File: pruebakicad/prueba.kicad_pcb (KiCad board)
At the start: 2 copper layers, 37 parts, among them J1 Conn_01x08_RC522, J2 Conn_01x04_MountingPin, J3 Conn_01x03, J4 Conn_2Rows-15Pins, J5 Conn_01x04, J6 Conn_01x02, Q1 BSS138, Q2 BSS138, U1 TLV1117-33, U2 TLV1117-50, U3 ESP32-WROOM-32

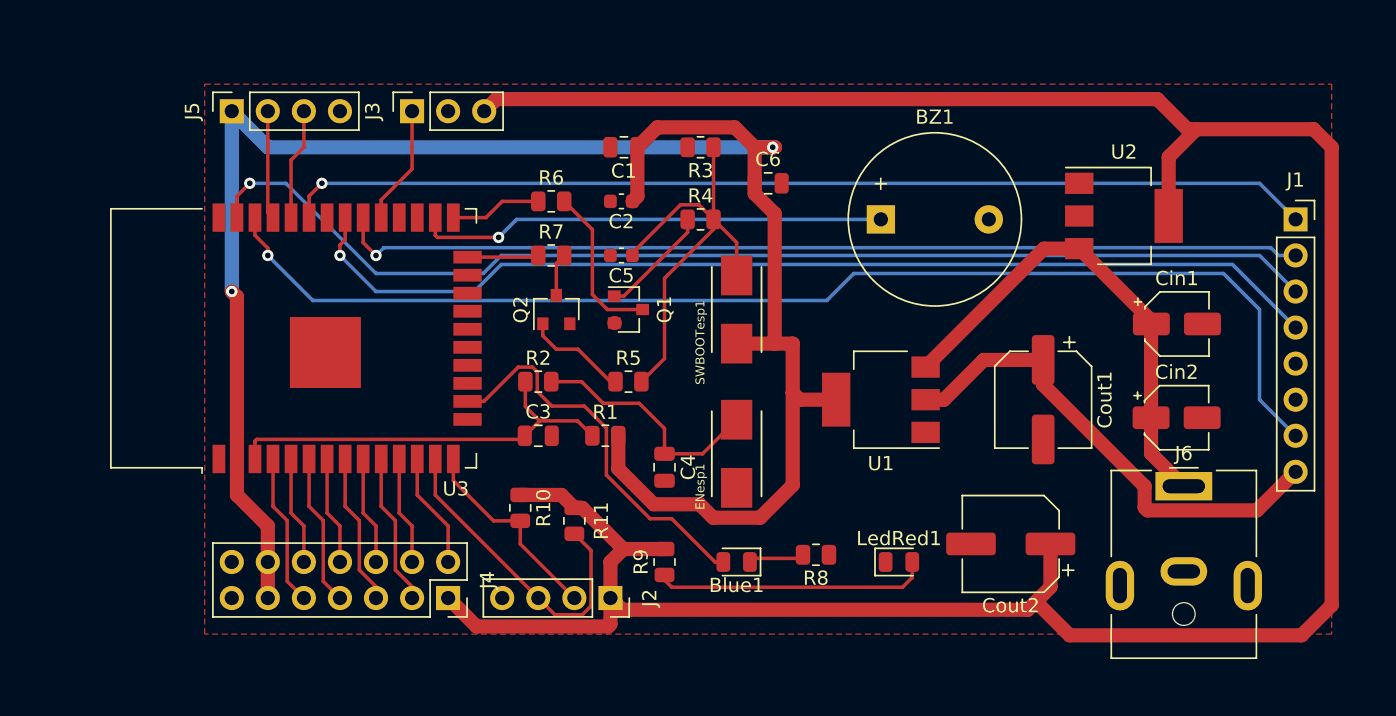
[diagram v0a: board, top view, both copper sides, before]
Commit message: tierras
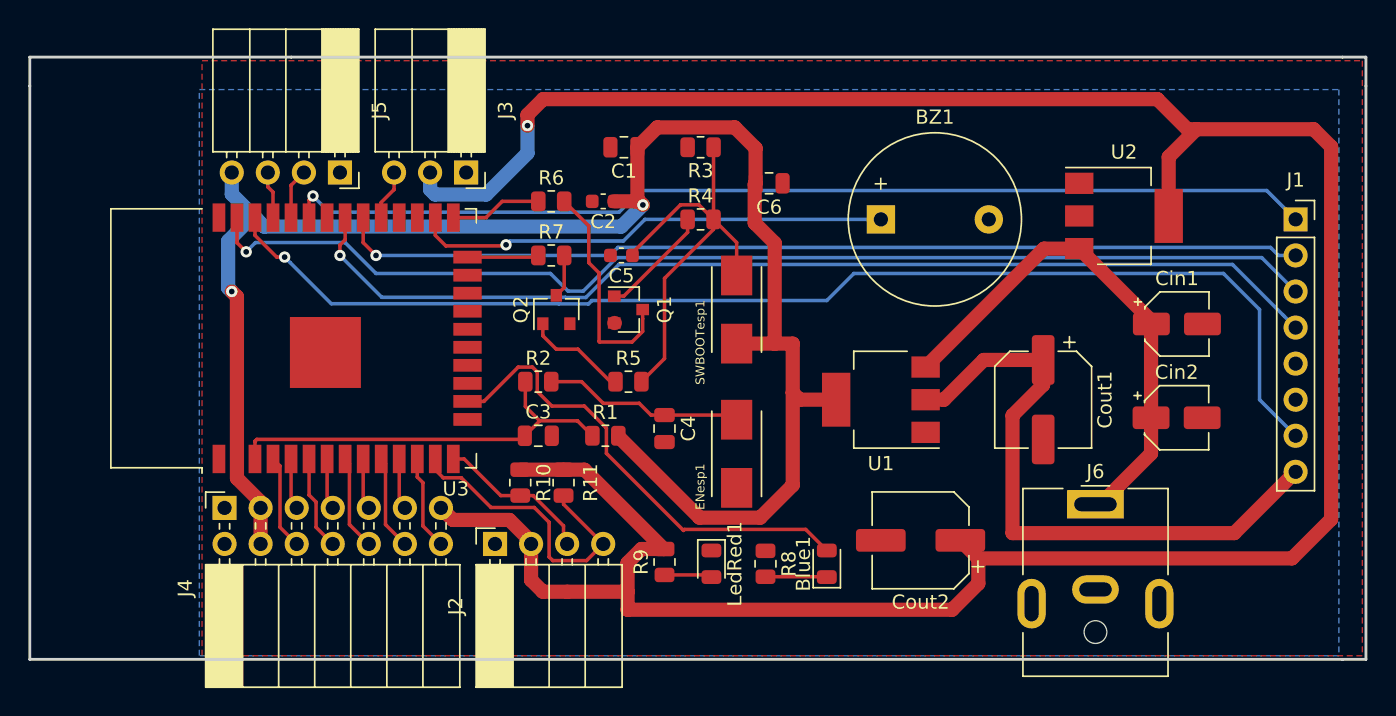
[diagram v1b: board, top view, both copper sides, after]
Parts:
- J2, J5: footprint Connector_PinSocket_2.54mm:PinSocket_1x04_P2.54mm_Vertical -> Connector_PinSocket_2.54mm:PinSocket_1x04_P2.54mm_Horizontal
- J3: footprint Connector_PinSocket_2.54mm:PinSocket_1x03_P2.54mm_Vertical -> Connector_PinSocket_2.54mm:PinSocket_1x03_P2.54mm_Horizontal
- J4: footprint Connector_PinSocket_2.54mm:PinSocket_2x07_P2.54mm_Vertical -> Connector_PinSocket_2.54mm:PinSocket_2x07_P2.54mm_Horizontal
- moved J4 17.0 mm to (42.7, 113.0), turned to 90 degrees
- moved LedRed1 13.2 mm to (77.0, 117.0), turned to 270 degrees
- moved J2 8.98 mm to (61.7, 115.6), turned to 90 degrees
- moved J5 8.76 mm to (50.8, 89.4), turned to 270 degrees
- moved Cout2 6.36 mm to (91.7, 115.3)
- moved Blue1 6.35 mm to (85.1, 117.0), turned to 90 degrees
- moved J6 6.35 mm to (104.0, 112.8)
- moved J3 5.76 mm to (59.7, 89.4), turned to 270 degrees
- moved R8 3.61 mm to (80.8, 117.0), turned to 270 degrees
- moved R11 2.80 mm to (66.5, 111.3)
- moved C4 2.73 mm to (73.7, 107.4)
- moved R10 1.78 mm to (63.5, 111.3)
- moved C2 1.28 mm to (69.3, 91.4)
- moved C6 0.07 mm to (81.0, 90.2), turned to 180 degrees
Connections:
- C6 pad 1: +3V3 -> GND
- C6 pad 2: GND -> +3V3
- J2 pad 1: +5V -> GND
- J2 pad 2: /SDAi2c -> +5V
- J2 pad 3: /SCLi2c -> /SDAi2c
- J2 pad 4: GND -> /SCLi2c
- J3 pad 1: /OBS -> GND
- J3 pad 2: GND -> +5V
- J3 pad 3: +5V -> /OBS
- J4 pad 1: +5V -> GND
- J4 pad 10: /sensVN -> /IO32
- J4 pad 11: +3V3 -> /IO26
- J4 pad 12: +3V3 -> /IO25
- J4 pad 13: GND -> +5V
- J4 pad 14: GND -> /IO27
- J4 pad 2: /IO27 -> GND
- J4 pad 3: /IO25 -> +3V3
- J4 pad 4: /IO26 -> +3V3
- J4 pad 5: /IO32 -> /sensVN
- J4 pad 6: /IO33 -> /sensVP
- J4 pad 7: /IO34 -> /IO35
- J4 pad 8: /IO35 -> /IO34
- J4 pad 9: /sensVP -> /IO33
- J5 pad 1: +3V3 -> GND
- J5 pad 2: /TXD0 -> /RXD0
- J5 pad 3: /RXD0 -> /TXD0
- J5 pad 4: GND -> +3V3
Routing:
- net Net-(LedRed1-Pad2): track 19.4 -> 3.72 mm
- net +3V3: track 172.7 -> 164.3 mm
- net +5V: track 188.1 -> 194.7 mm, vias 0 -> 1
- net /IO13: track 27.5 -> 33.6 mm
- net /OBS: track 8.40 -> 3.55 mm
- net Net-(Q1-Pad3): track 11.4 -> 15.8 mm
- net /TXD0: track 7.65 -> 3.33 mm
- net /RXD0: track 7.87 -> 3.55 mm
- net /sensVP: track 10.7 -> 6.68 mm
- net /IO34: track 10.7 -> 6.68 mm
- net /IO33: track 7.63 -> 3.61 mm
- net /IO26: track 7.63 -> 3.61 mm
- net /IO32: track 10.7 -> 6.68 mm
- net /IO25: track 10.7 -> 6.68 mm
- net /sensVN: track 7.63 -> 3.61 mm
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- added copper zone on B.Cu, net GND
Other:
- board outline added: 94.1 x 42.4 mm
